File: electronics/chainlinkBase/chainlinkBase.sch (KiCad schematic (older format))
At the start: 47 parts, among them J101 Power In, J102 RELAY, J103 Power In, J104 RS485, J105 RS485, J106 Logic Power Out, J107 UART, J108 Output, J109 Output, J110 Output, SW101 SW_DIP_x04, U101 AP7361C-33E, U102 TPL7407L, U103 Buck, U104 TTGO_TDisplay, U105 MCP23017_SS, U106 SN74LV1T34DBV, U107 SP485, U108 SN74LV1T34DBV

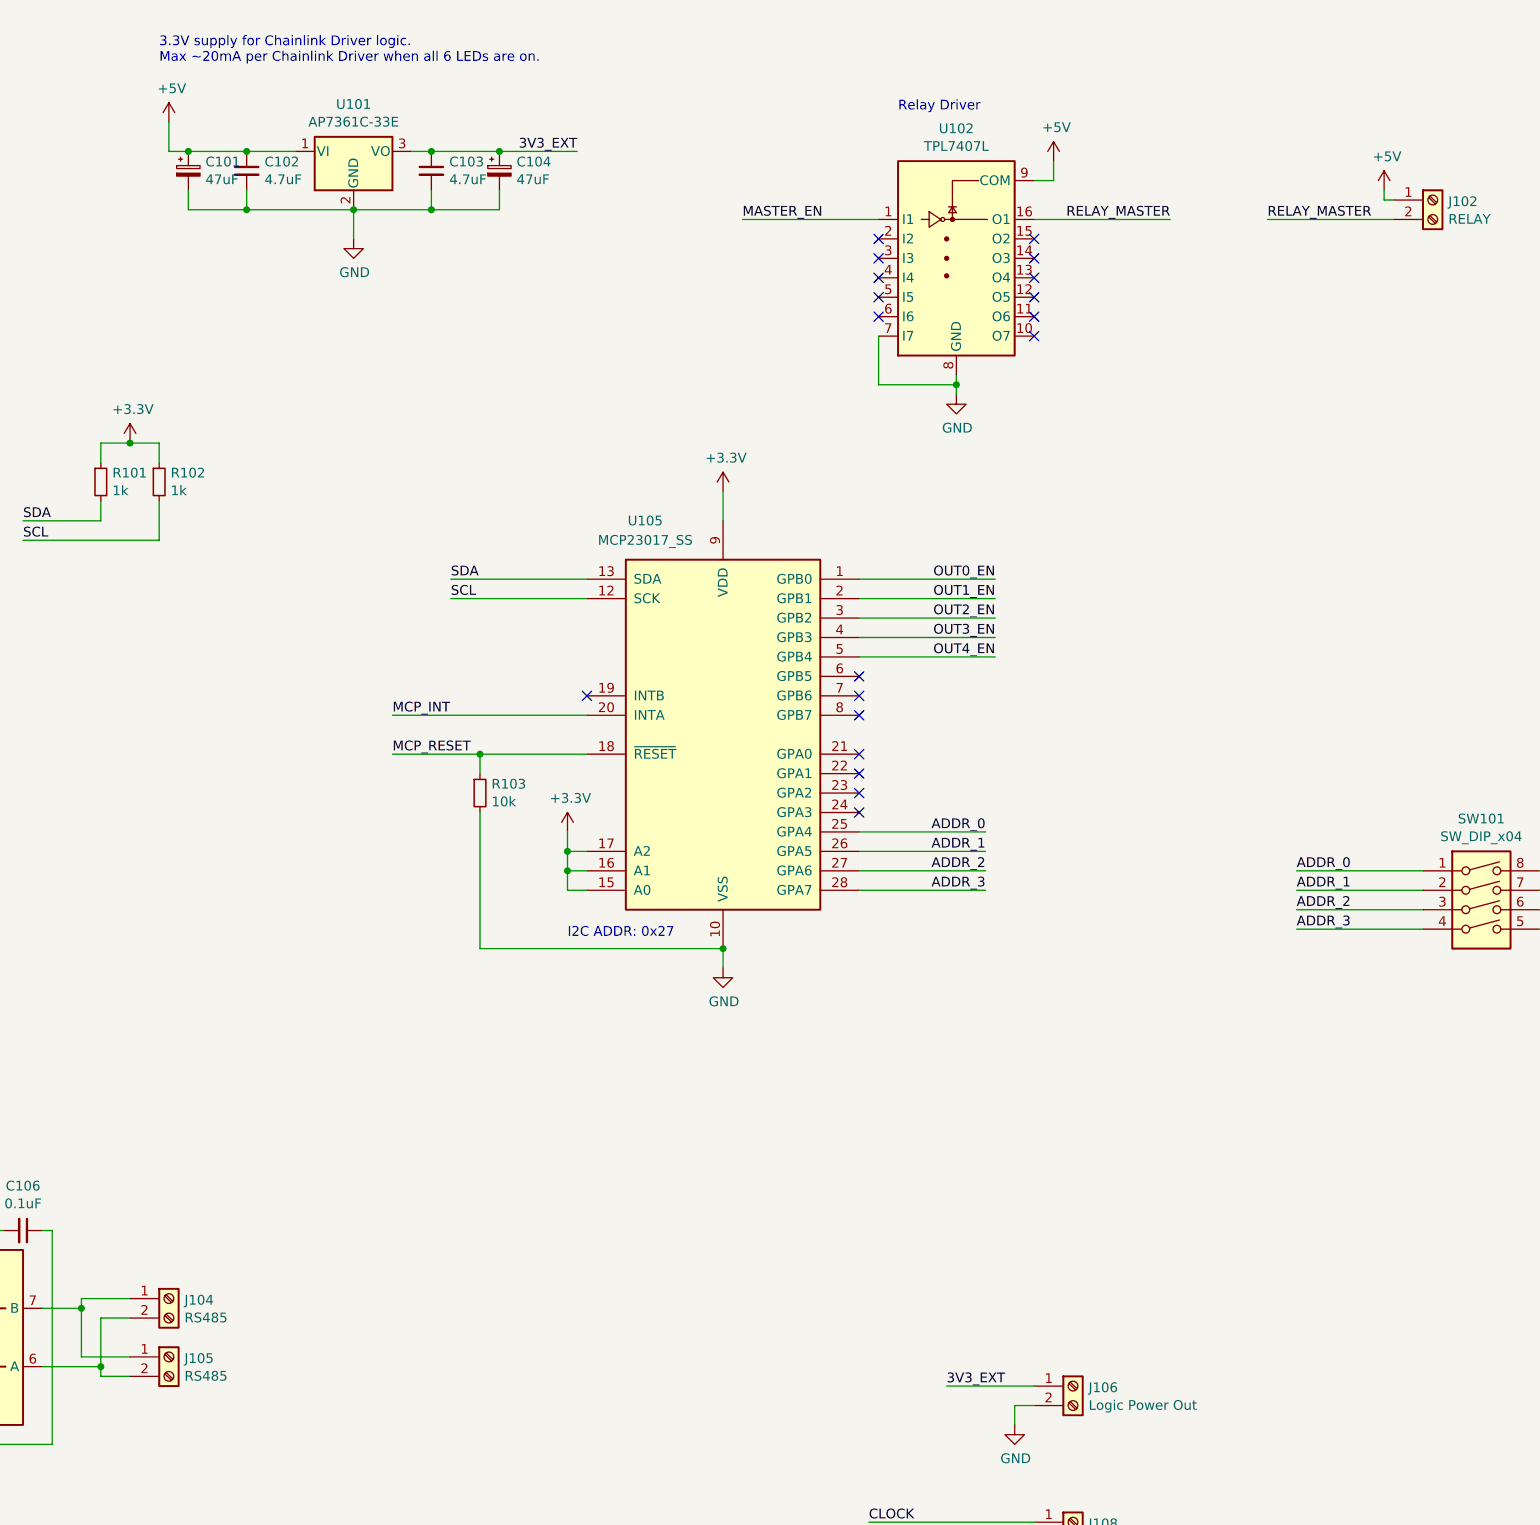
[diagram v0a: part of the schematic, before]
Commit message: Lots of layout and routing
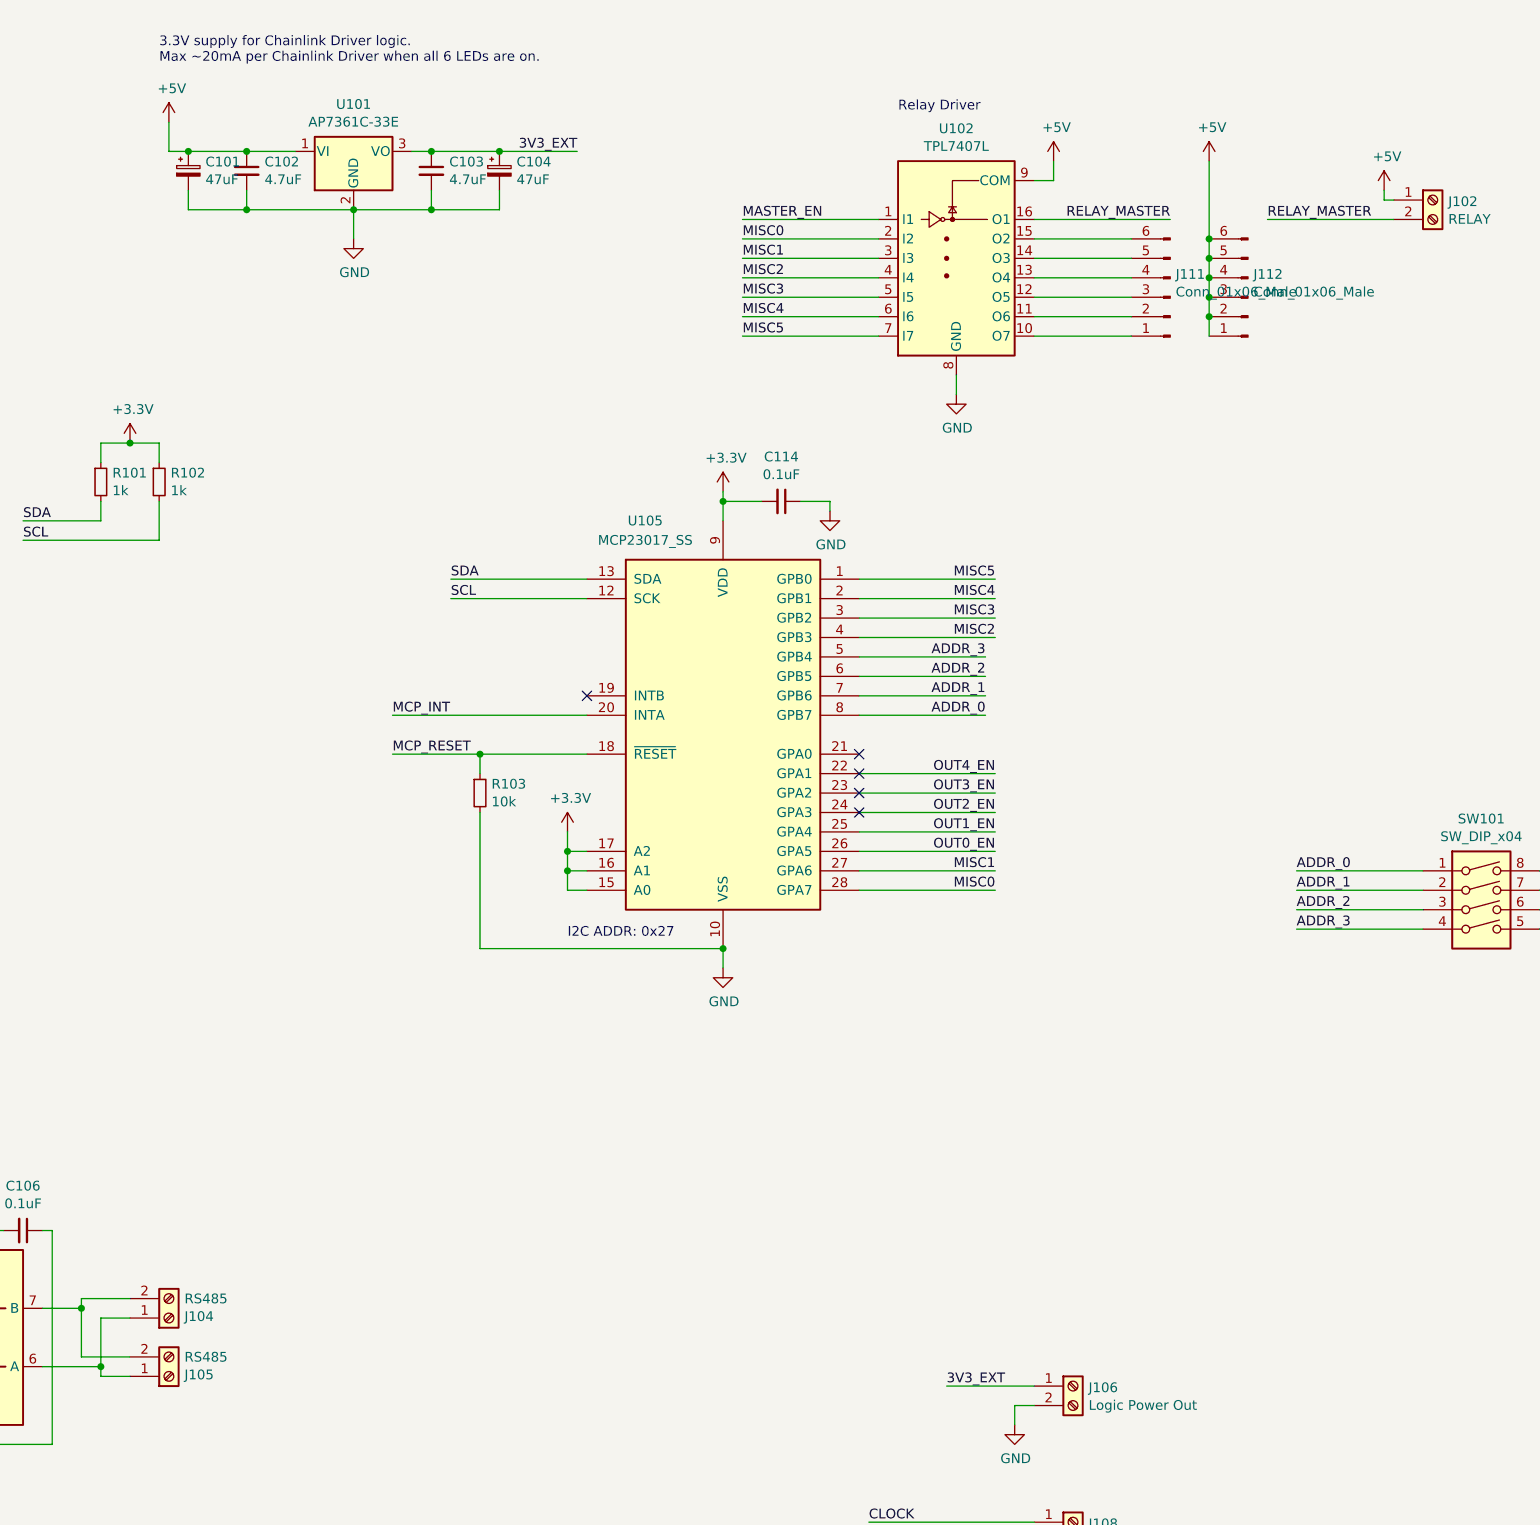
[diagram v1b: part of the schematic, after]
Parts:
- added C114: 0.1uF, Capacitor_SMD:C_0805_2012Metric, symbol Device:C_Small
- added J111, J112: Conn_01x06_Male, Connector_PinHeader_2.54mm:PinHeader_1x06_P2.54mm_Vertical, symbol Connector:Conn_01x06_Male
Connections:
- net +3V3: now also C114.2
- net +5V: now also J112.1 (Pin_1), J112.2 (Pin_2), J112.3 (Pin_3), J112.4 (Pin_4), J112.5 (Pin_5), J112.6 (Pin_6)
- net ADDR_0: now also U105.8 (GPB7); no longer U105.25 (GPA4)
- net ADDR_1: now also U105.7 (GPB6); no longer U105.26 (GPA5)
- net ADDR_2: now also U105.6 (GPB5); no longer U105.27 (GPA6)
- net ADDR_3: now also U105.5 (GPB4); no longer U105.28 (GPA7)
- net GND: now also C114.1; no longer U102.7 (I7)
- net OUT0_EN: now also U105.26 (GPA5); no longer U105.1 (GPB0)
- net OUT1_EN: now also U105.25 (GPA4); no longer U105.2 (GPB1)
- net OUT2_EN: now also U105.24 (GPA3); no longer U105.3 (GPB2)
- net OUT3_EN: now also U105.23 (GPA2); no longer U105.4 (GPB3)
- net OUT4_EN: now also U105.22 (GPA1); no longer U105.5 (GPB4)
- net at J104.2 (Pin_2), J105.2 (Pin_2): now also U107.7 (B); no longer U107.6 (A)
- net at J104.1 (Pin_1), J105.1 (Pin_1): now also U107.6 (A); no longer U107.7 (B)
- net at U102.10 (O7): now also J111.1 (Pin_1)
- net at U102.11 (O6): now also J111.2 (Pin_2)
- net at U102.12 (O5): now also J111.3 (Pin_3)
- net at U102.13 (O4): now also J111.4 (Pin_4)
- net at U102.14 (O3): now also J111.5 (Pin_5)
- net at U102.15 (O2): now also J111.6 (Pin_6)
- net MISC0: now reaches U102.2 (I2)
- net MISC0: now also U105.28 (GPA7)
- net MISC1: now reaches U102.3 (I3)
- net MISC1: now also U105.27 (GPA6)
- net MISC2: now reaches U102.4 (I4)
- net MISC2: now also U105.4 (GPB3)
- net MISC3: now reaches U102.5 (I5)
- net MISC3: now also U105.3 (GPB2)
- net MISC4: now reaches U102.6 (I6)
- net MISC4: now also U105.2 (GPB1)
- new net MISC5: U102.7 (I7), U105.1 (GPB0)
- no-connect marks 24 -> 10
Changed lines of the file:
@@
 L Connector:Screw_Terminal_01x02 J104
 U 1 1 60282EC9
-P 5200 7100
-F 0 "J104" H 5280 7092 50  0000 L CNN
-F 1 "RS485" H 5280 7001 50  0000 L CNN
-F 2 "ScrewTerminals:Generic-5.08-2P" H 5200 7100 50  0001 C CNN
-F 3 "~" H 5200 7100 50  0001 C CNN
-F 4 "EB147A-02-D" H 5200 7100 50  0001 C CNN "DK#"
-	1    5200 7100
-	1    0    0    -1
+P 5200 7200
+F 0 "J104" H 5280 7192 50  0000 L CNN
+F 1 "RS485" H 5280 7101 50  0000 L CNN
+F 2 "ScrewTerminals:Generic-5.08-2P" H 5200 7200 50  0001 C CNN
+F 3 "~" H 5200 7200 50  0001 C CNN
+F 4 "EB147A-02-D" H 5200 7200 50  0001 C CNN "DK#"
+	1    5200 7200
+	1    0    0    1
 $EndComp
 $Comp
 L Connector:Screw_Terminal_01x02 J105
 U 1 1 60284131
-P 5200 7400
-F 0 "J105" H 5280 7392 50  0000 L CNN
-F 1 "RS485" H 5280 7301 50  0000 L CNN
-F 2 "ScrewTerminals:Generic-5.08-2P" H 5200 7400 50  0001 C CNN
-F 3 "~" H 5200 7400 50  0001 C CNN
-F 4 "EB147A-02-D" H 5200 7400 50  0001 C CNN "DK#"
-	1    5200 7400
-	1    0    0    -1
+P 5200 7500
+F 0 "J105" H 5280 7492 50  0000 L CNN
+F 1 "RS485" H 5280 7401 50  0000 L CNN
+F 2 "ScrewTerminals:Generic-5.08-2P" H 5200 7500 50  0001 C CNN
+F 3 "~" H 5200 7500 50  0001 C CNN
+F 4 "EB147A-02-D" H 5200 7500 50  0001 C CNN "DK#"
+	1    5200 7500
+	1    0    0    1
 $EndComp
 Wire Wire Line
@@
 	6650 3400 7350 3400
 Wire Wire Line
-	8750 3400 9450 3400
-Text Label 9450 3400 2    50   ~ 0
+	8750 4800 9450 4800
+Text Label 9450 4800 2    50   ~ 0
 OUT0_EN
 Wire Wire Line
-	8750 3500 9450 3500
-Text Label 9450 3500 2    50   ~ 0
+	8750 4700 9450 4700
+Text Label 9450 4700 2    50   ~ 0
 OUT1_EN
 Wire Wire Line
-	8750 3700 9450 3700
-Text Label 9450 3700 2    50   ~ 0
+	8750 4500 9450 4500
+Text Label 9450 4500 2    50   ~ 0
 OUT3_EN
 Wire Wire Line
-	8750 3800 9450 3800
-Text Label 9450 3800 2    50   ~ 0
+	8750 4400 9450 4400
+Text Label 9450 4400 2    50   ~ 0
 OUT4_EN
 $Comp
@@
 $EndComp
 Wire Wire Line
-	8050 3100 8050 2950
+	8050 3100 8050 3000
 $Comp
 L power:+3.3V #PWR0123
@@
 	1    0    0    -1
 $EndComp
-Wire Wire Line
-	9250 2350 9250 2400
 $Comp
 L power:+5V #PWR0139
@@
 	1    0    0    -1
 $EndComp
-Wire Wire Line
-	8850 2400 9250 2400
-Wire Wire Line
-	8850 2150 8850 2400
-Connection ~ 9250 2400
-Wire Wire Line
-	9250 2400 9250 2450
 Wire Wire Line
 	8850 1550 8150 1550
@@
 Text Notes 17350 2450 0    50   ~ 0
 I2C ADDR: 0x40
-NoConn ~ 9650 2150
 Wire Wire Line
 	1500 10550 2550 10550
@@
 ADDR_3
 Wire Wire Line
-	9400 4700 8750 4700
-Wire Wire Line
-	8750 4800 9400 4800
-Wire Wire Line
-	9400 4900 8750 4900
-Wire Wire Line
-	8750 5000 9400 5000
-Text Label 9400 4700 2    50   ~ 0
+	9400 4100 8750 4100
+Wire Wire Line
+	8750 4000 9400 4000
+Wire Wire Line
+	9400 3900 8750 3900
+Wire Wire Line
+	8750 3800 9400 3800
+Text Label 9400 4100 2    50   ~ 0
 ADDR_0
-Text Label 9400 4800 2    50   ~ 0
+Text Label 9400 4000 2    50   ~ 0
 ADDR_1
-Text Label 9400 4900 2    50   ~ 0
+Text Label 9400 3900 2    50   ~ 0
 ADDR_2
-Text Label 9400 5000 2    50   ~ 0
+Text Label 9400 3800 2    50   ~ 0
 ADDR_3
 NoConn ~ 8750 4500
@@
 $EndComp
 Connection ~ 3500 3550
-$Comp
-L Transistor_Array:ULN2003A U102
-U 1 1 60BF5C71
-P 9250 1750
-F 0 "U102" H 9250 2417 50  0000 C CNN
-F 1 "TPL7407L" H 9250 2326 50  0000 C CNN
-F 2 "ModifiedSymbols:SOIC-16_3.9x9.9mm_P1.27mm_silk" H 9300 1200 50  0001 L CNN
-F 3 "" H 9350 1550 50  0001 C CNN
-F 4 "296-51862-1-ND" H 9250 1750 50  0001 C CNN "DK#"
-	1    9250 1750
-	1    0    0    -1
-$EndComp
 Text Label 10850 1550 0    50   ~ 0
 RELAY_MASTER
@@
 Wire Wire Line
 	11450 1450 11500 1450
-NoConn ~ 9650 1650
-NoConn ~ 9650 1750
-NoConn ~ 9650 1850
-NoConn ~ 9650 1950
-NoConn ~ 9650 2050
-NoConn ~ 8850 2050
-NoConn ~ 8850 1950
-NoConn ~ 8850 1850
-NoConn ~ 8850 1750
-NoConn ~ 8850 1650
-Text Label 9450 3600 2    50   ~ 0
+Text Label 9450 4600 2    50   ~ 0
 OUT2_EN
 Wire Wire Line
-	8750 3600 9450 3600
-NoConn ~ 8750 3900
-NoConn ~ 8750 4000
-NoConn ~ 8750 4100
+	8750 4600 9450 4600
 NoConn ~ 8750 4300
 NoConn ~ 8750 4400
@@
 	17650 6350 17650 6450
 $Comp
-L power:GND #PWR?
+L power:GND #PWR0142
 U 1 1 606F96E9
 P 13100 950
-F 0 "#PWR?" H 13100 700 50  0001 C CNN
+F 0 "#PWR0142" H 13100 700 50  0001 C CNN
 F 1 "GND" H 13105 777 50  0000 C CNN
 F 2 "" H 13100 950 50  0001 C CNN
@@
 Wire Wire Line
 	13100 850  13200 850
+$Comp
+L Connector:Conn_01x06_Male J111
+U 1 1 607902DC
+P 10350 1950
+F 0 "J111" H 10322 1832 50  0000 R CNN
+F 1 "Conn_01x06_Male" H 10322 1923 50  0000 R CNN
+F 2 "Connector_PinHeader_2.54mm:PinHeader_1x06_P2.54mm_Vertical" H 10350 1950 50  0001 C CNN
+F 3 "~" H 10350 1950 50  0001 C CNN
+	1    10350 1950
+	-1   0    0    1
+$EndComp
+Wire Wire Line
+	9650 1650 10150 1650
+Wire Wire Line
+	9650 1750 10150 1750
+Wire Wire Line
+	9650 1850 10150 1850
+Wire Wire Line
+	9650 1950 10150 1950
+Wire Wire Line
+	9650 2050 10150 2050
+Wire Wire Line
+	9650 2150 10150 2150
+$Comp
+L Connector:Conn_01x06_Male J112
+U 1 1 6082E04D
+P 10750 1950
+F 0 "J112" H 10722 1832 50  0000 R CNN
+F 1 "Conn_01x06_Male" H 10722 1923 50  0000 R CNN
+F 2 "Connector_PinHeader_2.54mm:PinHeader_1x06_P2.54mm_Vertical" H 10750 1950 50  0001 C CNN
+F 3 "~" H 10750 1950 50  0001 C CNN
+	1    10750 1950
+	-1   0    0    1
+$EndComp
+$Comp
+L power:+5V #PWR0143
+U 1 1 6082EB4F
+P 10550 1250
+F 0 "#PWR0143" H 10550 1100 50  0001 C CNN
+F 1 "+5V" H 10565 1423 50  0000 C CNN
+F 2 "" H 10550 1250 50  0001 C CNN
+F 3 "" H 10550 1250 50  0001 C CNN
+	1    10550 1250
+	1    0    0    -1
+$EndComp
+Wire Wire Line
+	10550 1250 10550 1650
+Connection ~ 10550 1650
+Wire Wire Line
+	10550 1650 10550 1750
+Connection ~ 10550 1750
+Wire Wire Line
+	10550 1750 10550 1850
+Connection ~ 10550 1850
+Wire Wire Line
+	10550 1850 10550 1950
+Connection ~ 10550 1950
+Wire Wire Line
+	10550 1950 10550 2050
+Connection ~ 10550 2050
+Wire Wire Line
+	10550 2050 10550 2150
+Wire Wire Line
+	9250 2350 9250 2450
+Wire Wire Line
+	8850 2150 8150 2150
+Text Label 8150 2150 0    50   ~ 0
+MISC5
+Wire Wire Line
+	8850 2050 8150 2050
+Text Label 8150 2050 0    50   ~ 0
+MISC4
+Wire Wire Line
+	8850 1950 8150 1950
+Text Label 8150 1950 0    50   ~ 0
+MISC3
+Wire Wire Line
+	8850 1850 8150 1850
+Text Label 8150 1850 0    50   ~ 0
+MISC2
+Wire Wire Line
+	8850 1750 8150 1750
+Text Label 8150 1750 0    50   ~ 0
+MISC1
+Wire Wire Line
+	8850 1650 8150 1650
+Text Label 8150 1650 0    50   ~ 0
+MISC0
+Wire Wire Line
+	9450 3400 8750 3400
+Text Label 9450 3400 2    50   ~ 0
+MISC5
+Wire Wire Line
+	9450 3500 8750 3500
+Text Label 9450 3500 2    50   ~ 0
+MISC4
+Wire Wire Line
+	9450 3600 8750 3600
+Text Label 9450 3600 2    50   ~ 0
+MISC3
+Wire Wire Line
+	9450 3700 8750 3700
+Text Label 9450 3700 2    50   ~ 0
+MISC2
+Wire Wire Line
+	9450 4900 8750 4900
+Text Label 9450 4900 2    50   ~ 0
+MISC1
+Wire Wire Line
+	9450 5000 8750 5000
+Text Label 9450 5000 2    50   ~ 0
+MISC0
+$Comp
+L Transistor_Array:ULN2003A U102
+U 1 1 60BF5C71
+P 9250 1750
+F 0 "U102" H 9250 2417 50  0000 C CNN
+F 1 "TPL7407L" H 9250 2326 50  0000 C CNN
+F 2 "ModifiedSymbols:SOIC-16_3.9x9.9mm_P1.27mm_silk" H 9300 1200 50  0001 L CNN
+F 3 "" H 9350 1550 50  0001 C CNN
+F 4 "296-51862-1-ND" H 9250 1750 50  0001 C CNN "DK#"
+	1    9250 1750
+	1    0    0    -1
+$EndComp
+$Comp
+L Device:C_Small C114
+U 1 1 60A2AB1E
+P 8350 3000
+F 0 "C114" V 8121 3000 50  0000 C CNN
+F 1 "0.1uF" V 8212 3000 50  0000 C CNN
+F 2 "Capacitor_SMD:C_0805_2012Metric" H 8350 3000 50  0001 C CNN
+F 3 "~" H 8350 3000 50  0001 C CNN
+	1    8350 3000
+	0    1    1    0
+$EndComp
+$Comp
+L power:GND #PWR0144
+U 1 1 60A2C0EA
+P 8600 3050
+F 0 "#PWR0144" H 8600 2800 50  0001 C CNN
+F 1 "GND" H 8605 2877 50  0000 C CNN
+F 2 "" H 8600 3050 50  0001 C CNN
+F 3 "" H 8600 3050 50  0001 C CNN
+	1    8600 3050
+	1    0    0    -1
+$EndComp
+Wire Wire Line
+	8450 3000 8600 3000
+Wire Wire Line
+	8600 3000 8600 3050
+Wire Wire Line
+	8250 3000 8050 3000
+Connection ~ 8050 3000
+Wire Wire Line
+	8050 3000 8050 2950
 $EndSCHEMATC
